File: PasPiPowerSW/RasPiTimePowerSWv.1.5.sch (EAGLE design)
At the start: 38 parts, among them IC1 MSP430G2553, IC2 NJM2845DL1-33, J1 3P Socket, J2 3P Socket, Q1 P-ch MOS FET, T1 2SC1815-Y

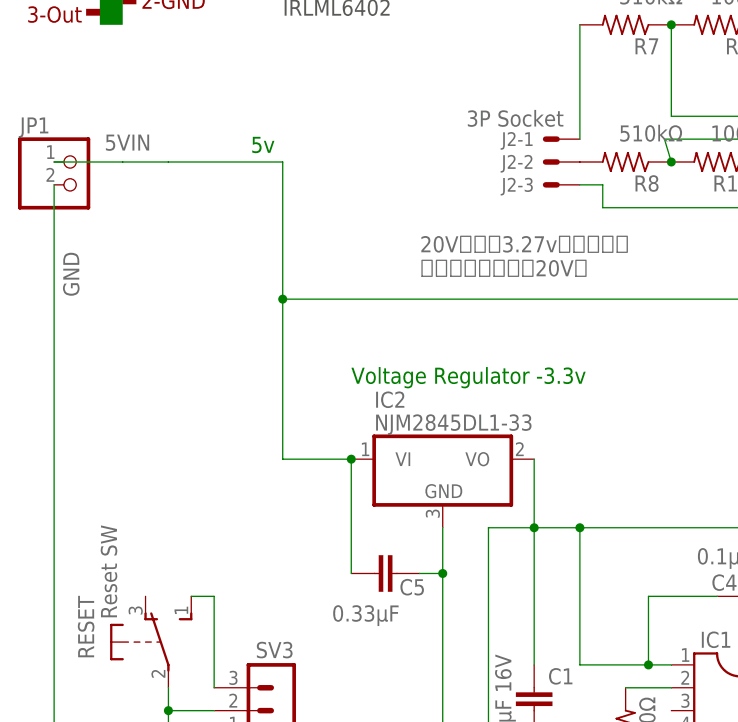
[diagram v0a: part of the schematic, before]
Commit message: Replaced TO-252 Voltage Regulator part
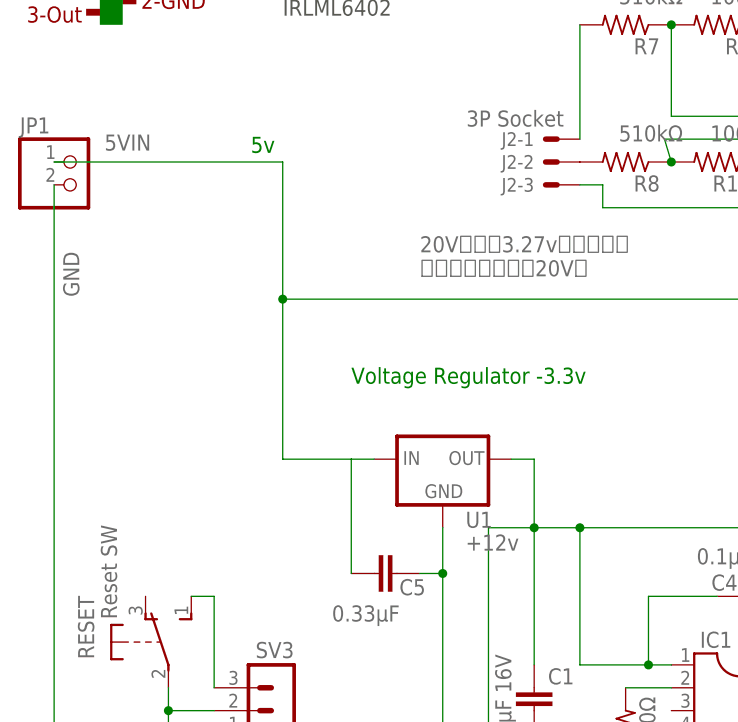
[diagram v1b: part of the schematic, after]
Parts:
- removed IC2: NJM2845DL1-33, linear:7818DT
- added U1: +12v, SparkFun-IC-Power:V_REG_78XX7812
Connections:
- net 3.3V: now also U1.OUT; no longer IC2.VO
- net 5VIN: now also U1.IN; no longer IC2.VI
- net GND: now also U1.GND; no longer IC2.GND

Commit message: Revert "revert to NJM2845DL1"
This reverts commit ec86f7a8aa55efb6e9586fa3a205028523492dc4.
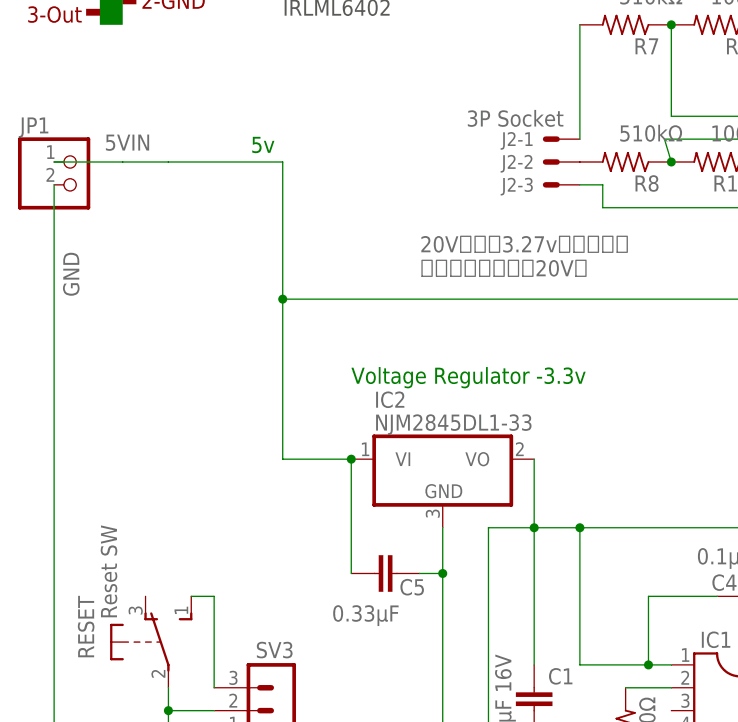
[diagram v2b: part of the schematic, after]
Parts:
- removed U1: +12v, SparkFun-IC-Power:V_REG_78XX7812
- added IC2: NJM2845DL1-33, linear:7818DT
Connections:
- net 3.3V: now also IC2.VO; no longer U1.OUT
- net 5VIN: now also IC2.VI; no longer U1.IN
- net GND: now also IC2.GND; no longer U1.GND
